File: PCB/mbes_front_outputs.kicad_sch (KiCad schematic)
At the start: 55 parts, among them Q1 BC817, Q11 TPCA8120,L1Q, Q14 BC817, Q15 BC817, Q19 BC817, Q2 BC817, Q20 BC817, Q21 BC817, Q3 BC817, Q4 TPCA8120,L1Q, Q5 TPCA8120,L1Q, Q6 TPCA8120,L1Q, Q7 TPCA8120,L1Q, Q8 TPCA8120,L1Q

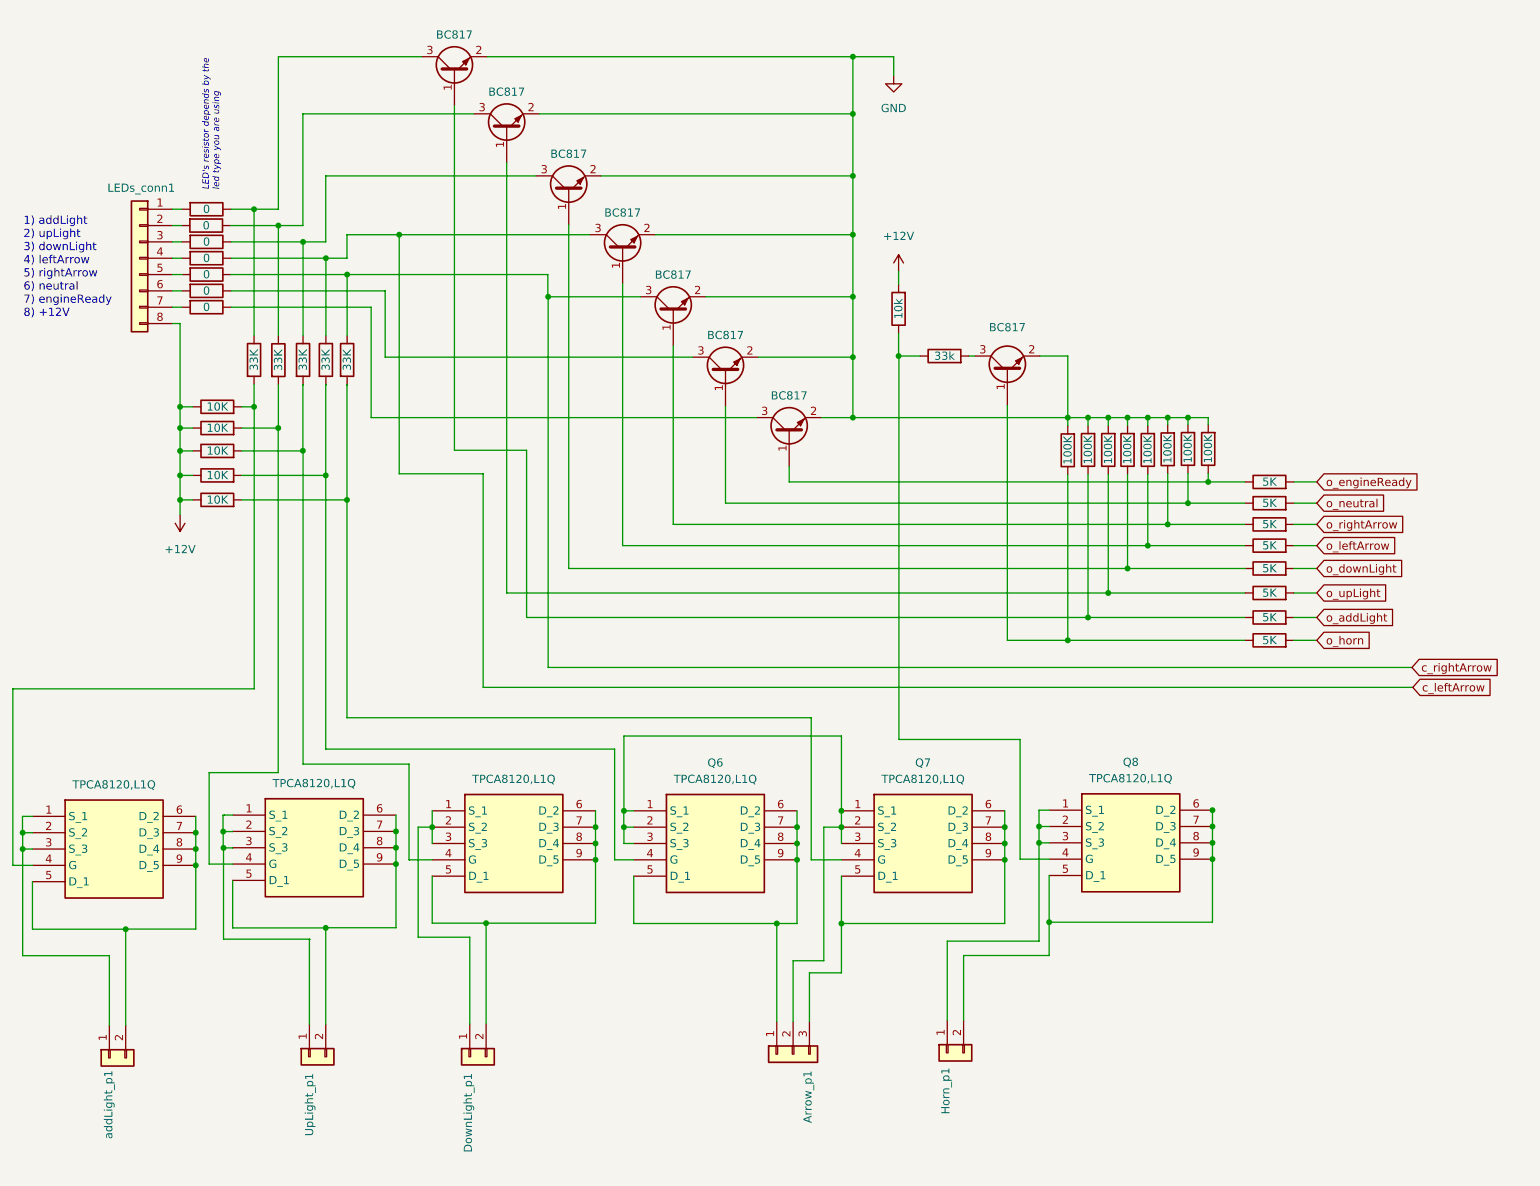
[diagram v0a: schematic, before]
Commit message: Manual merging from the ATmega16__dualPCB branch
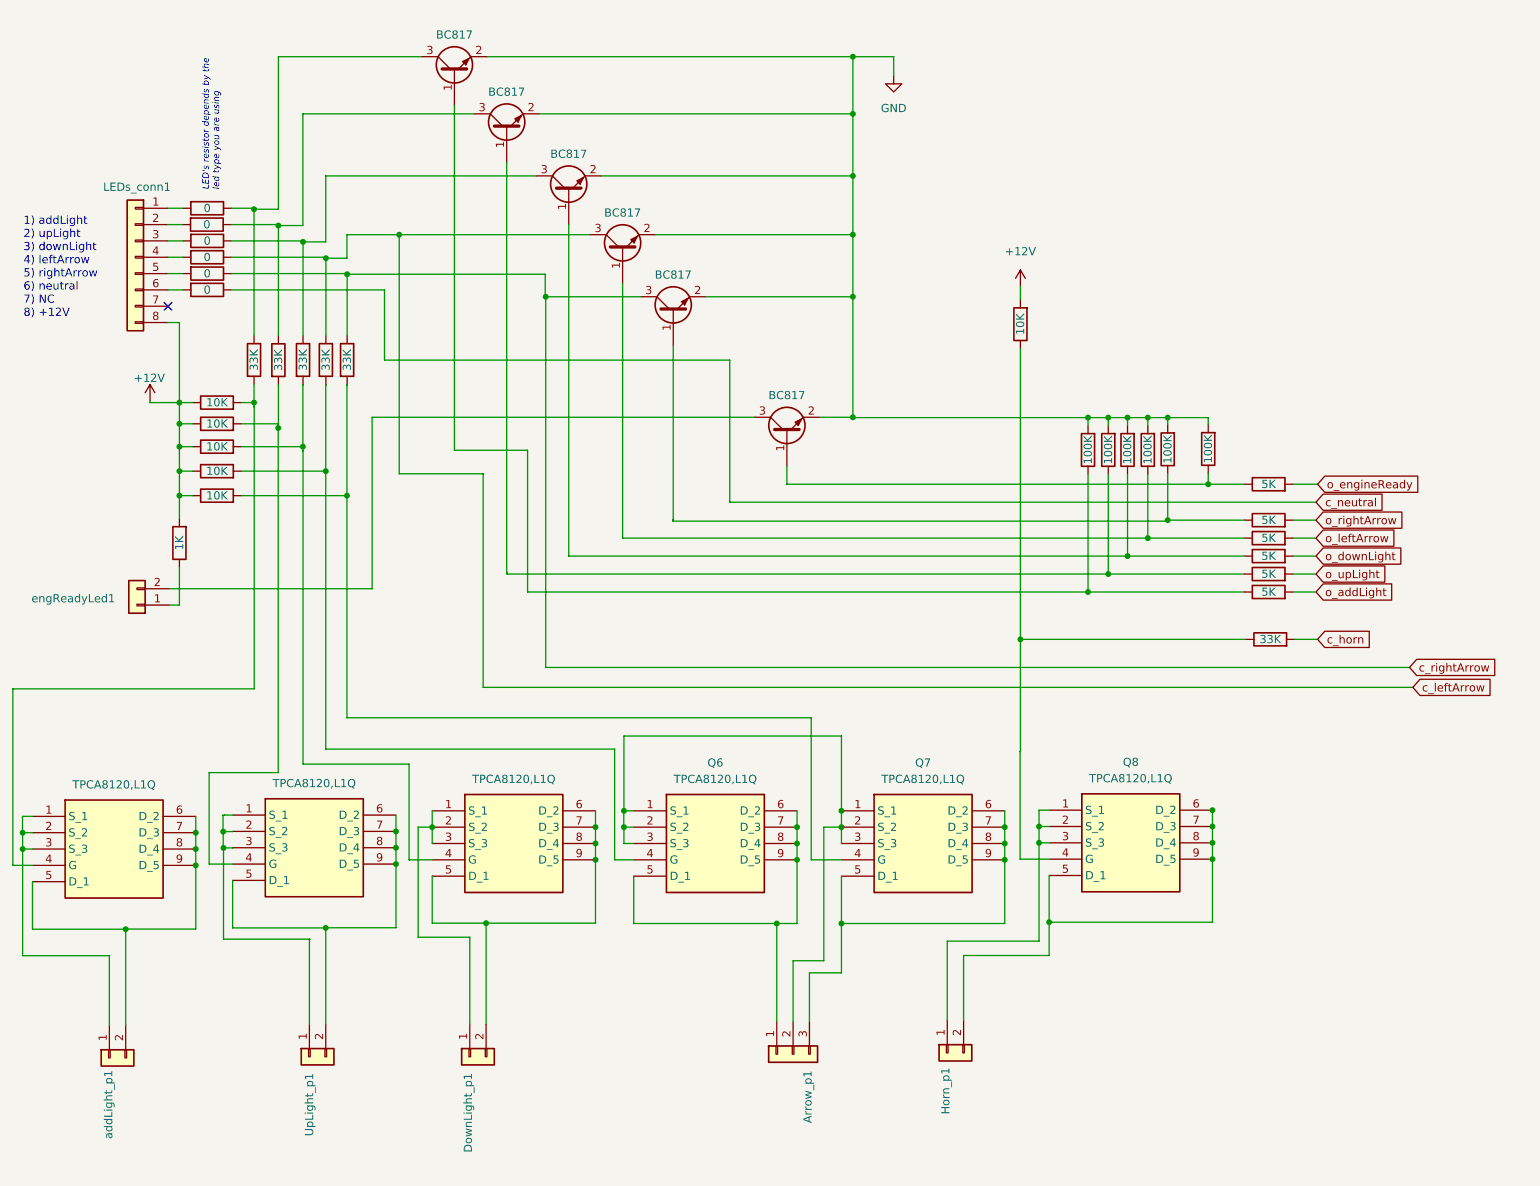
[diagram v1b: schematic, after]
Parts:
- removed Q20, Q3: BC817, Package_TO_SOT_SMD:SOT-23, symbol Transistor_BJT:BC817
- removed RA15: 33k, Resistor_SMD:R_1206_3216Metric, symbol Device:R
- removed RA17: 5K, Resistor_SMD:R_1206_3216Metric, symbol Device:R
- removed RA32, RA39: 100K, Resistor_SMD:R_1206_3216Metric, symbol Device:R
- added engReadyLed1: Conn_01x02, Connector_PinHeader_2.54mm:PinHeader_1x02_P2.54mm_Vertical, symbol Connector_Generic:Conn_01x02
- LEDs_conn1: footprint Connector_PinHeader_2.54mm:PinHeader_1x08_P2.54mm_Vertical -> Connector_PinHeader_2.54mm:PinHeader_2x04_P2.54mm_Vertical
- RA42: value 10k -> 10K
- RA7: value 5K -> 33K
- RA9: value 0 -> 1K
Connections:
- net +12V: now also RA9.2
- net at RA7.1: now also Q8.4 (G), RA42.1
- net at Q21.3 (C): now also engReadyLed1.2 (Pin_2); no longer RA9.1
- net at LEDs_conn1.7 (Pin_7): no longer RA9.2
- net c_neutral: now reaches RA6.1
- net o_horn renamed c_horn
- new net: RA9.1, engReadyLed1.1 (Pin_1)
- no-connect marks 0 -> 1
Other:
- note added: "1) addLight 2) upLight 3) downLight 4) leftArrow 5) rightArrow 6) neutral 7) NC 8) +12V"
- note removed: "1) addLight 2) upLight 3) downLight 4) leftArrow 5) rightArrow 6) neutral 7) engineReady 8) +12V"
- moved on the sheet: LEDs_conn1

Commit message: Old files replaced.
They have been merged for error
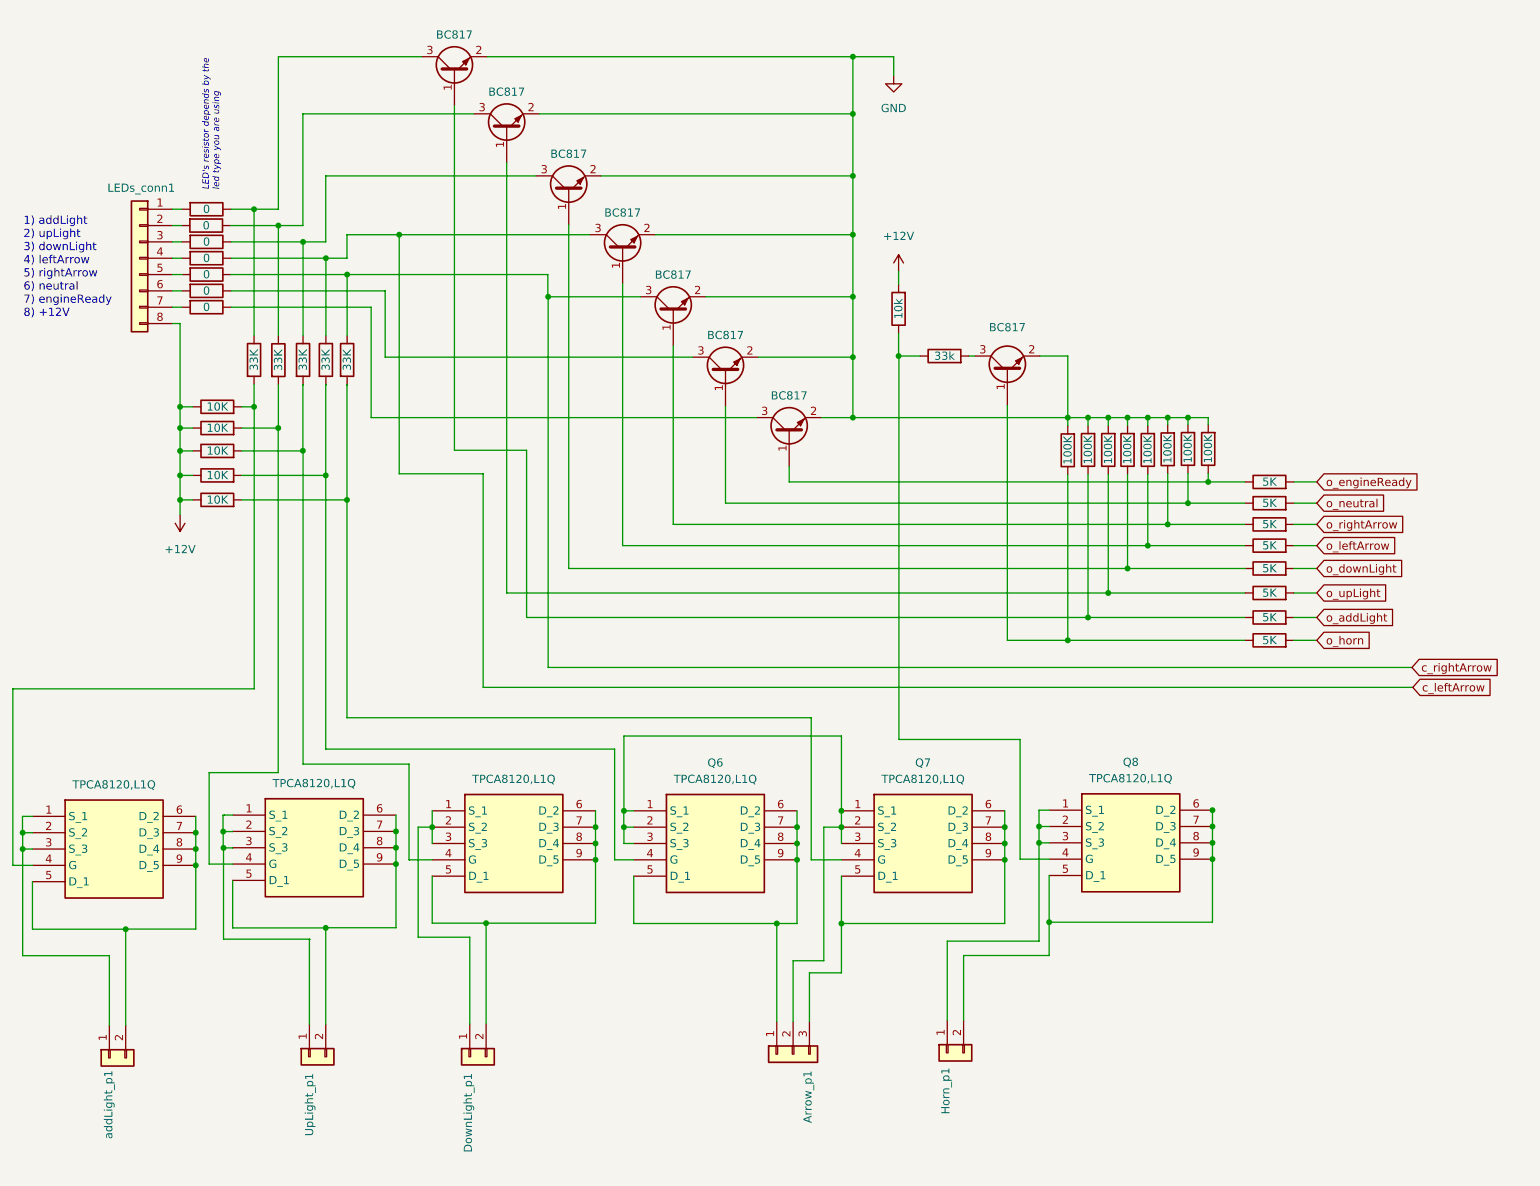
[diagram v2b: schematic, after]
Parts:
- removed engReadyLed1: Conn_01x02, Connector_PinHeader_2.54mm:PinHeader_1x02_P2.54mm_Vertical, symbol Connector_Generic:Conn_01x02
- added Q20, Q3: BC817, Package_TO_SOT_SMD:SOT-23, symbol Transistor_BJT:BC817
- added RA15: 33k, Resistor_SMD:R_1206_3216Metric, symbol Device:R
- added RA17: 5K, Resistor_SMD:R_1206_3216Metric, symbol Device:R
- added RA32, RA39: 100K, Resistor_SMD:R_1206_3216Metric, symbol Device:R
- LEDs_conn1: footprint Connector_PinHeader_2.54mm:PinHeader_2x04_P2.54mm_Vertical -> Connector_PinHeader_2.54mm:PinHeader_1x08_P2.54mm_Vertical
- RA42: value 10K -> 10k
- RA7: value 33K -> 5K
- RA9: value 1K -> 0
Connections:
- net +12V: no longer RA9.2
- net GND: now also Q20.2 (E), Q3.2 (E), RA32.2, RA39.2
- net at Q21.3 (C): now also RA9.1
- net at LEDs_conn1.7 (Pin_7): now also RA9.2
- net at Q8.4 (G), RA42.1: now also RA15.1; no longer RA7.1
- net c_horn renamed o_horn
- net c_neutral: no longer names the net of RA6.1
- net c_neutral: now also Q20.3 (C)
- new net: Q3.1 (B), RA32.1, RA7.1
- new net: Q3.3 (C), RA15.2
- new net: Q20.1 (B), RA17.1, RA39.1
- new net o_neutral: RA17.2
- no-connect marks 1 -> 0
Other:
- note added: "1) addLight 2) upLight 3) downLight 4) leftArrow 5) rightArrow 6) neutral 7) engineReady 8) +12V"
- note removed: "1) addLight 2) upLight 3) downLight 4) leftArrow 5) rightArrow 6) neutral 7) NC 8) +12V"
- moved on the sheet: LEDs_conn1
